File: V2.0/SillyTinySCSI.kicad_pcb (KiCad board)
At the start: 4 copper layers, 53.5 x 25 mm, 65 parts, among them J1 DB25_Plug, J2 Micro_SD_Card_Det1, U1 74LVT125, U2 74LVT245, U3 74LVT125, U4 74LVT245, U5 TLV75728PDBVR, U6 Pico W

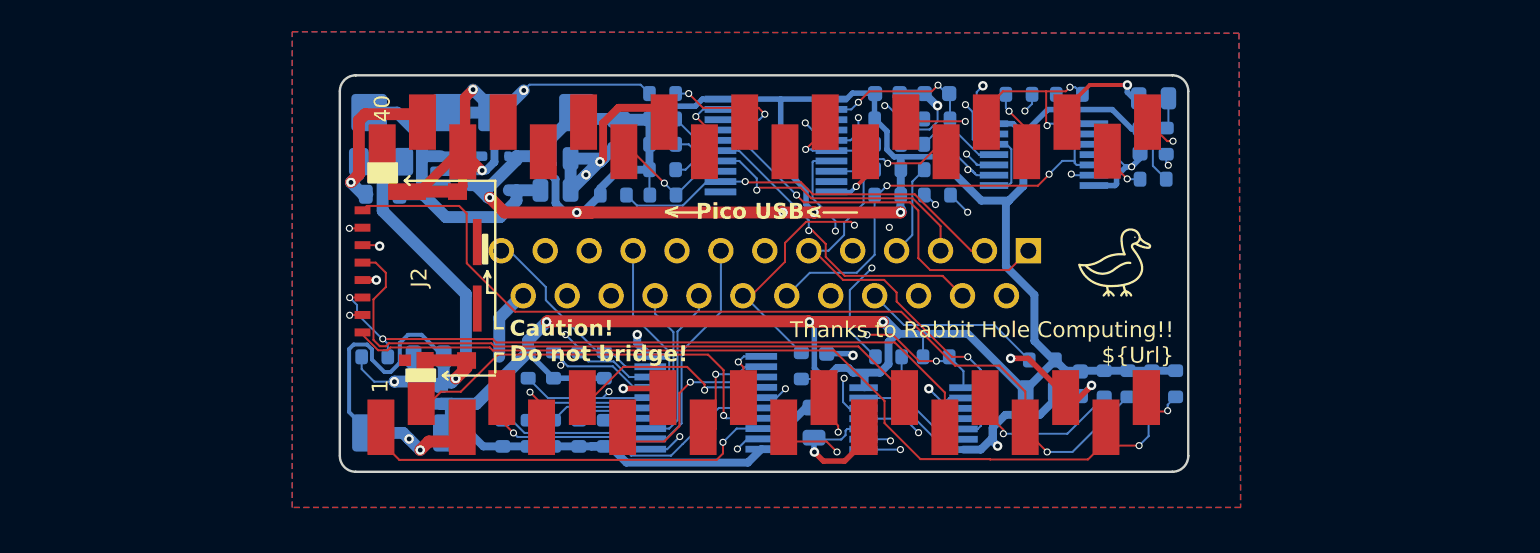
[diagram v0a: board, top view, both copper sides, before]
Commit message: Initial version of Centronics 50 SillyTinySCSI
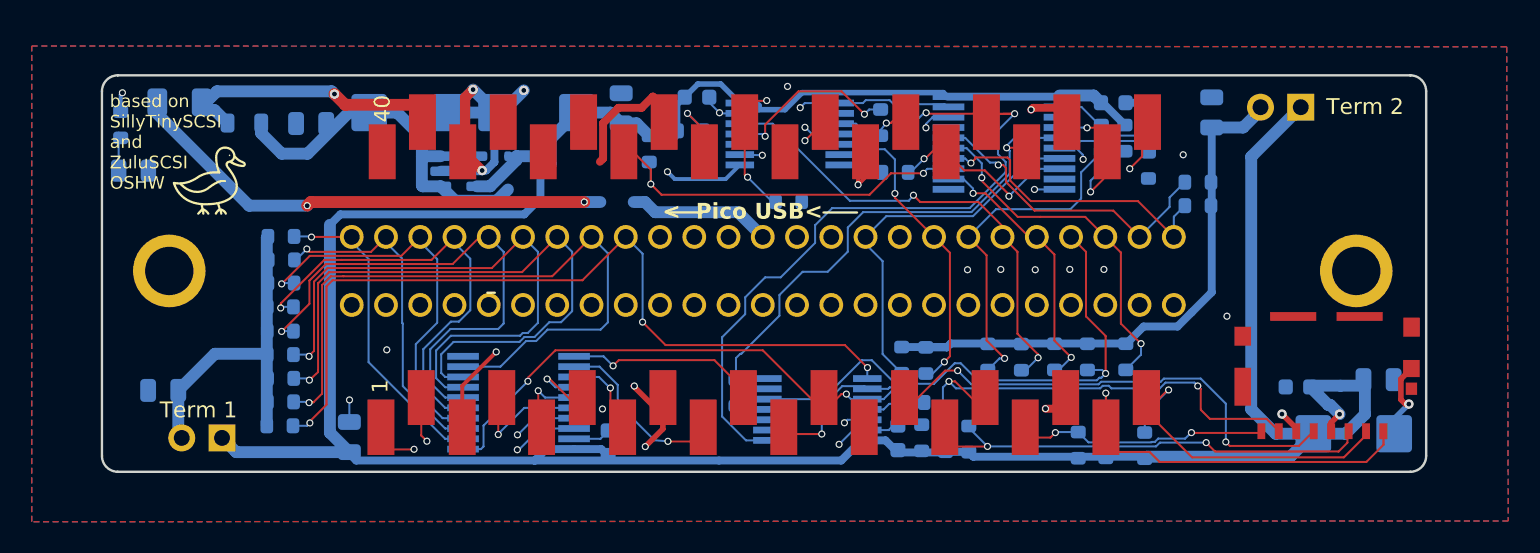
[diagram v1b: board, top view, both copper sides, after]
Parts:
- added JP1: Term 1, Connector_PinHeader_2.54mm:PinHeader_1x02_P2.54mm_Vertical, B.Cu at (100.6, 73.1)
- added JP2: Term 2, Connector_PinHeader_2.54mm:PinHeader_1x02_P2.54mm_Vertical, B.Cu at (168.6, 52.3)
- J1: value DB25_Plug -> Centronics50_Plug; footprint ZuluSCSI:DSUB-25_Male_Vertical_Small Courtyard -> Centronics:111050113L001
- moved R15 65.9 mm to (94.2, 53.4), turned to 90 degrees
- moved D3 64.5 mm to (95.0, 56.3), turned to 180 degrees
- moved C12 59.9 mm to (173.5, 69.4)
- moved C9 59.5 mm to (171.9, 72.8), turned to 0 degrees
- moved J2 57.5 mm to (170.2, 69.1), turned to 0 degrees
- moved G*** 57.3 mm to (99.8, 56.9)
- moved C13 54.8 mm to (168.4, 69.9), turned to 0 degrees
- moved C3 43.7 mm to (108.6, 73.1), turned to 90 degrees
- moved J1 42.8 mm to (108.8, 64.7), turned to 0 degrees
- moved R16 37.8 mm to (147.7, 73.2), turned to -90 degrees
- moved R11 34.0 mm to (162.1, 57.0), turned to 0 degrees
- moved R8 33.8 mm to (162.1, 58.5), turned to 0 degrees
- moved R12 33.1 mm to (104.2, 72.3), turned to 180 degrees
- moved C15 33.0 mm to (96.9, 70.1), turned to 180 degrees
- moved R10 32.1 mm to (157.6, 68.0), turned to 90 degrees
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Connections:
- C14 pad 1: +2V8 -> Net-(JP2-B)
- C15 pad 1: +2V8 -> Net-(JP1-B)
- J1 pad 1: ~{SCSI_REQ} -> GND
- J1 pad 10: ~{SCSI_DB3} -> GND
- J1 pad 11: ~{SCSI_DB5} -> GND
- J1 pad 12: ~{SCSI_DB6} -> unconnected-(J1-Pad12)
- J1 pad 13: ~{SCSI_DB7} -> unconnected-(J1-Pad13)
- J1 pad 14: GND -> unconnected-(J1-Pad14)
- J1 pad 15: ~{SCSI_CD} -> GND
- J1 pad 17: ~{SCSI_ATN} -> GND
- J1 pad 19: ~{SCSI_SEL} -> GND
- J1 pad 2: ~{SCSI_MSG} -> GND
- J1 pad 20: ~{SCSI_DBP} -> GND
- J1 pad 21: ~{SCSI_DB1} -> GND
- J1 pad 22: ~{SCSI_DB2} -> GND
- J1 pad 23: ~{SCSI_DB4} -> GND
- J1 pad 25: TERMPWR_5V -> GND
- J1 pad 3: ~{SCSI_IO} -> GND
- J1 pad 4: ~{SCSI_RST} -> GND
- J1 pad 5: ~{SCSI_ACK} -> GND
- J1 pad 6: ~{SCSI_BSY} -> GND
- J1 pad 8: ~{SCSI_DB0} -> GND
- R10 pad 2: +2V8 -> Net-(JP2-B)
- R11 pad 2: +2V8 -> Net-(JP2-B)
- R12 pad 2: +2V8 -> Net-(JP1-B)
- R13 pad 2: +2V8 -> Net-(JP2-B)
- R14 pad 2: +2V8 -> Net-(JP2-B)
- R21 pad 2: +2V8 -> Net-(JP2-B)
- R22 pad 2: +2V8 -> Net-(JP2-B)
- R23 pad 2: +2V8 -> Net-(JP2-B)
- R24 pad 2: +2V8 -> Net-(JP1-B)
- R25 pad 2: +2V8 -> Net-(JP1-B)
- R26 pad 2: +2V8 -> Net-(JP1-B)
- R27 pad 2: +2V8 -> Net-(JP1-B)
- R28 pad 2: +2V8 -> Net-(JP1-B)
- R29 pad 2: +2V8 -> Net-(JP1-B)
- R3 pad 2: +2V8 -> Net-(JP2-B)
- R30 pad 2: +2V8 -> Net-(JP1-B)
- R31 pad 2: +2V8 -> Net-(JP1-B)
- R8 pad 2: +2V8 -> Net-(JP2-B)
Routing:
- net +2V8: track 299.0 -> 195.7 mm, vias 10 -> 1
- net GND: track 159.8 -> 77.0 mm, vias 24 -> 26
- net /cpu/SDIO_D1: track 59.2 -> 16.5 mm, vias 1 -> 2
- net /cpu/SDIO_D3: track 62.7 -> 23.7 mm, vias 2 -> 1
- net Net-(JP2-B): track 0.00 -> 36.4 mm
- net ~{OUT_SEL}: track 12.0 -> 45.9 mm
- net /cpu/SDIO_D0: track 62.8 -> 31.2 mm
- net ~{SCSI_DB7}: track 12.4 -> 43.7 mm, vias 0 -> 1
- net /cpu/SDIO_D2: track 56.6 -> 25.9 mm
- net ~{SCSI_DB6}: track 12.2 -> 41.3 mm
- net ~{SCSI_DB5}: track 15.3 -> 37.3 mm
- net Net-(JP1-B): track 0.00 -> 21.8 mm
- net ~{SCSI_DBP}: track 36.8 -> 58.5 mm, vias 2 -> 4
- net ~{GPIO_IO}: track 7.68 -> 28.0 mm, vias 1 -> 2
- net ~{SCSI_DB4}: track 14.9 -> 33.2 mm
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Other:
- board size 53.5 x 25 mm -> 83.5 x 25 mm
- board text added: "Term 1"
- board text added: "Term 2"
- board text added: "based on SillyTinySCSI and ZuluSCSI OSHW"
- board text removed: "Caution! Do not bridge!"
- board text removed: "SillyTinySCSI"
- board text removed: "Thanks to Rabbit Hole Computing!! ${Url}"
- board text removed: "ZZJ"
- board text removed: "ZuluSCSI OSHW"
